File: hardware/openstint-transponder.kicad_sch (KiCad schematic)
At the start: 33 parts, among them J1 V+, J2 V-, Q1 AO3401A, U1 STM32C011F4Ux, U3 UCC27517DBV, U4 TLV760xx, Y1 20 MHz

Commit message: readme update
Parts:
- R3: LCSC (none) -> C17168
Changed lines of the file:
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@@
+			)
+		)
+		(property "LCSC" "C17168"
+			(at 180.34 140.97 90)
+			(effects
+				(font
+					(size 1.27 1.27)
+				)
+				(hide yes)
 			)
 		)

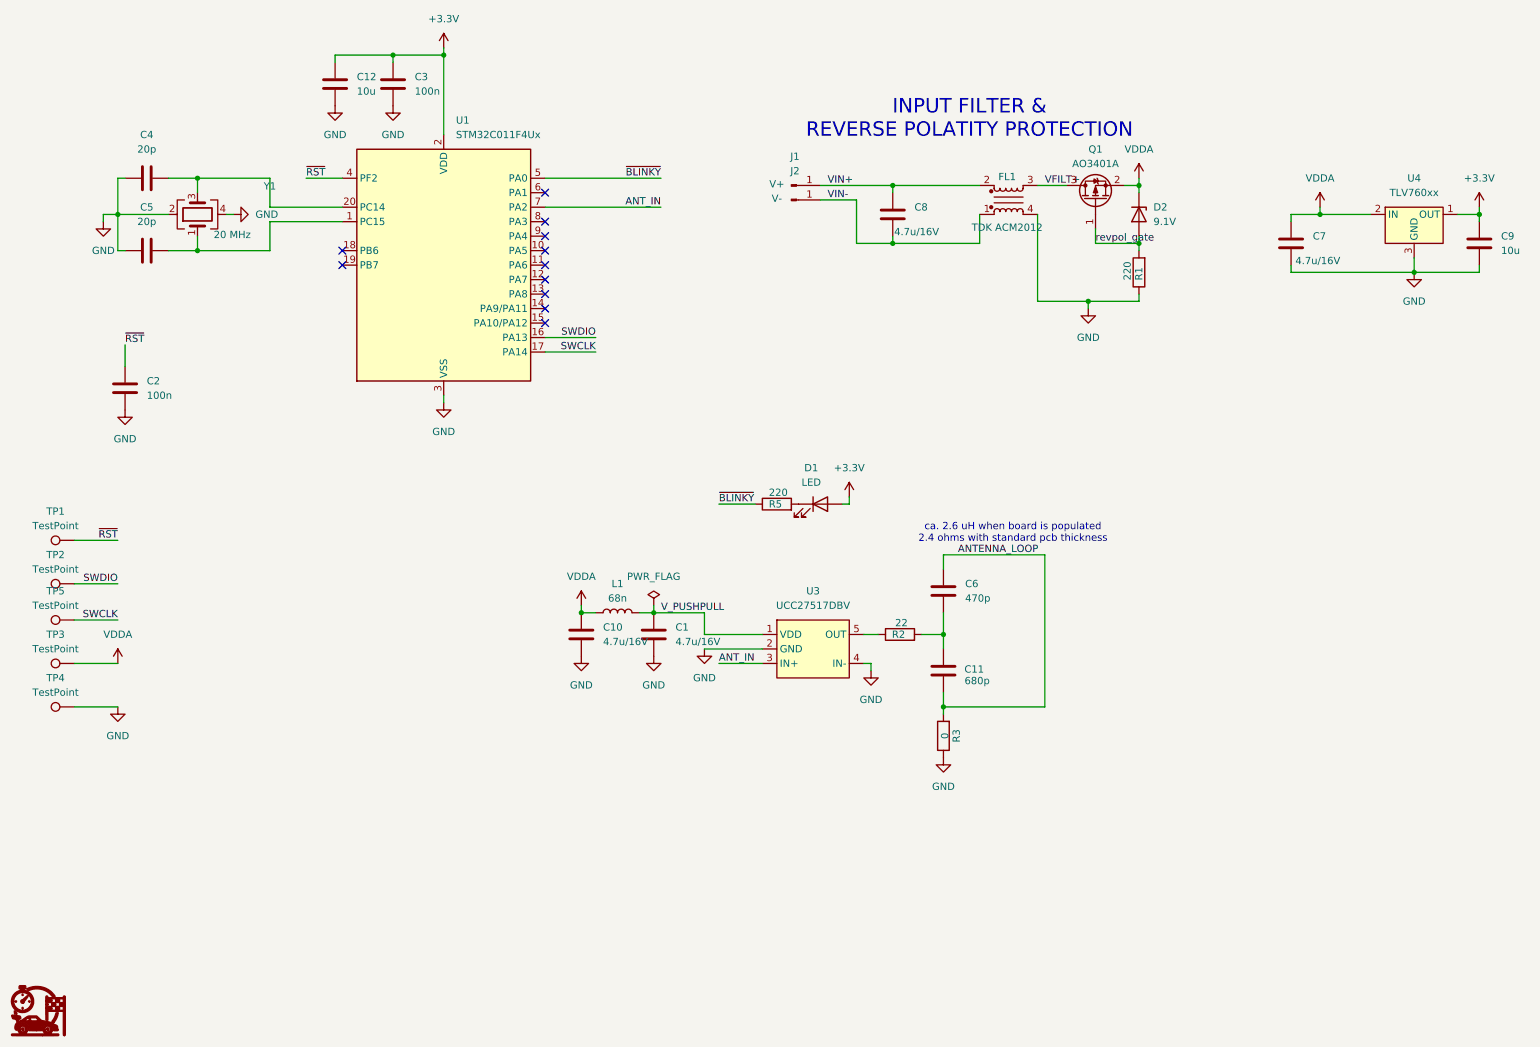
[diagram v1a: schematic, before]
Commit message: v2 transponder
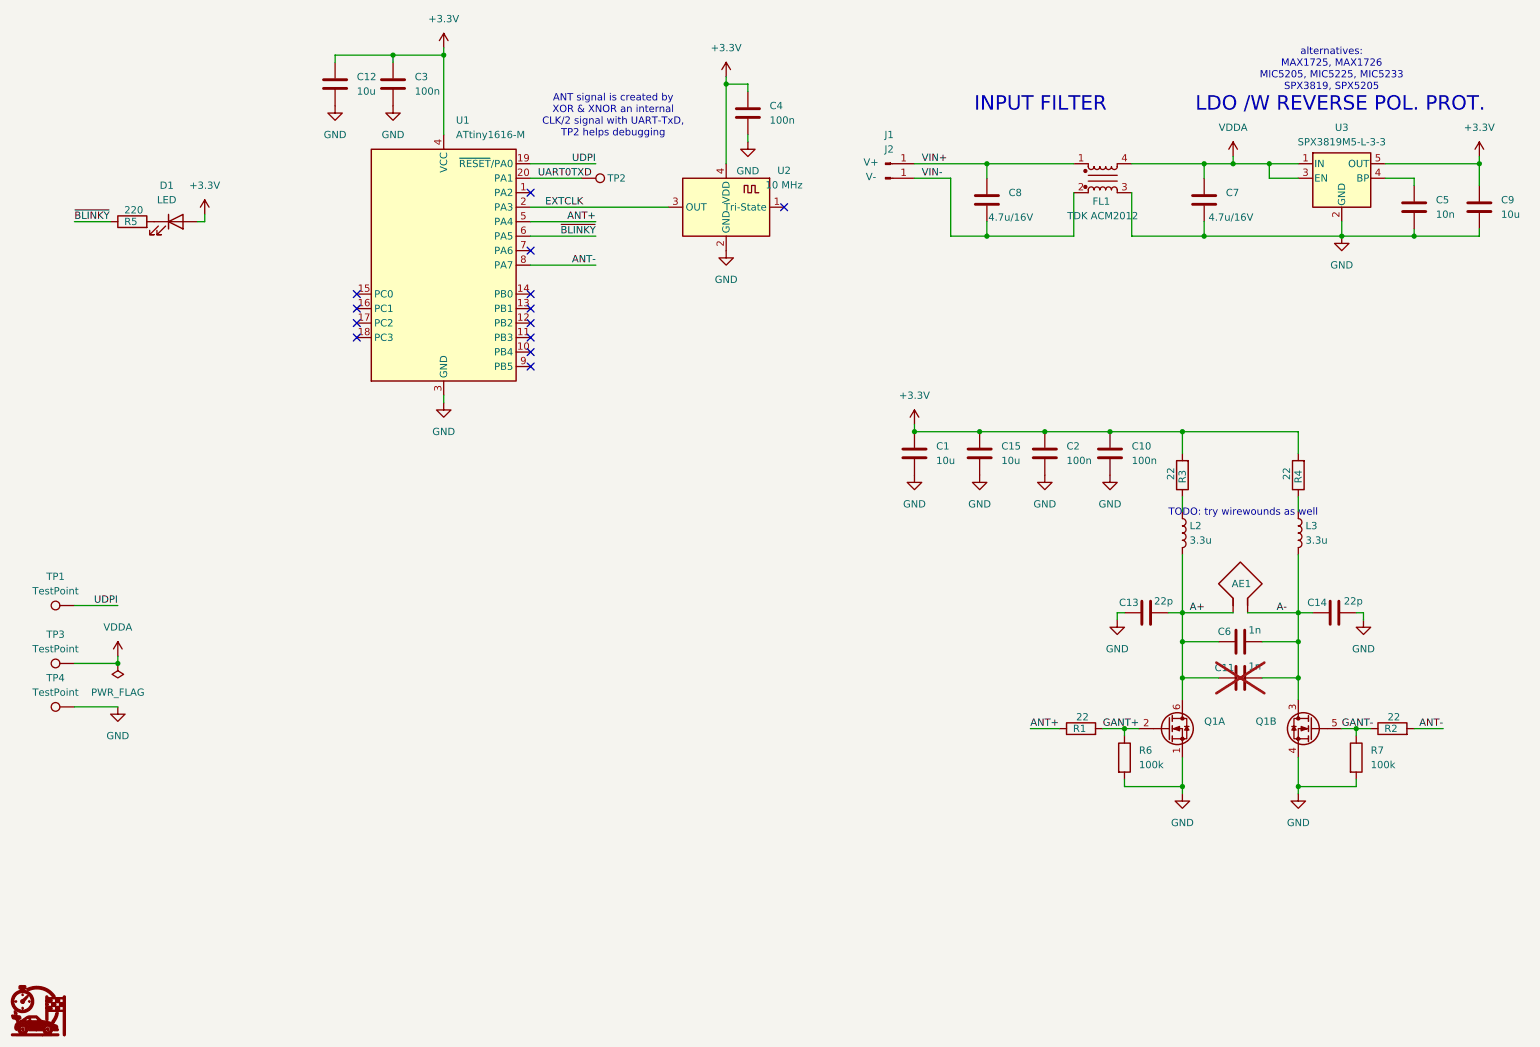
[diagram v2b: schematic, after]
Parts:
- removed D2: 9.1V, Diode_SMD:D_SOD-323, symbol Device:D_Zener
- removed L1: 68n, Inductor_SMD:L_0603_1608Metric, symbol Device:L
- removed Q1: AO3401A, Package_TO_SOT_SMD:SOT-23, symbol Transistor_FET:AO3401A
- removed TP5: TestPoint, TestPoint:TestPoint_Pad_D1.0mm, symbol Connector:TestPoint
- removed U1: STM32C011F4Ux, Package_DFN_QFN:ST_UFQFPN-20_3x3mm_P0.5mm, symbol MCU_ST_STM32C0:STM32C011F4Ux
- removed U3: UCC27517DBV, Package_TO_SOT_SMD:SOT-23-5, symbol Driver_FET:UCC27517DBV
- removed U4: TLV760xx, Package_TO_SOT_SMD:SOT-23, symbol Regulator_Linear:TLV760xx
- removed Y1: 20 MHz, Crystal:Crystal_SMD_3225-4Pin_3.2x2.5mm, symbol Device:Crystal_GND24
- added AE1: Antenna_Loop, symbol Device:Antenna_Loop
- added C13, C14: 22p, Capacitor_SMD:C_0402_1005Metric, symbol Device:C
- added C15: 10u, Capacitor_SMD:C_0402_1005Metric, symbol Device:C
- added L2, L3: 3.3u, Inductor_SMD:L_0603_1608Metric, symbol Device:L
- added Q1: PMGD280UN, Package_TO_SOT_SMD:SOT-363_SC-70-6, symbol Transistor_FET:Q_Dual_NMOS_S1G1D2S2G2D1
- added R4: 22, Resistor_SMD:R_0402_1005Metric, symbol Device:R
- added R6, R7: 100k, Resistor_SMD:R_0402_1005Metric, symbol Device:R
- added U1: ATtiny1616-M, Package_DFN_QFN:VQFN-20-1EP_3x3mm_P0.4mm_EP1.7x1.7mm, symbol MCU_Microchip_ATtiny:ATtiny1616-M
- added U2: 10 MHz, Crystal:Crystal_SMD_3225-4Pin_3.2x2.5mm, symbol symbols:Oscillator
- added U3: SPX3819M5-L-3-3, Package_TO_SOT_SMD:SOT-23-5, symbol Regulator_Linear:SPX3819M5-L-3-3
- C1: value 4.7u/16V -> 10u; footprint Capacitor_SMD:C_0603_1608Metric -> Capacitor_SMD:C_0402_1005Metric; LCSC C19666 -> C15525
- C10: value 4.7u/16V -> 100n; footprint Capacitor_SMD:C_0603_1608Metric -> Capacitor_SMD:C_0402_1005Metric; LCSC C19666 -> C1525
- C11: value 680p -> 1n; footprint Capacitor_SMD:C_0603_1608Metric -> Capacitor_SMD:C_0402_1005Metric; LCSC C30816 -> C1523; now not fitted
- C4: value 20p -> 100n; LCSC C1554 -> C1525
- C5: value 20p -> 10n; LCSC C1554 -> C15195
- C6: value 470p -> 1n; footprint Capacitor_SMD:C_0603_1608Metric -> Capacitor_SMD:C_0402_1005Metric; LCSC C1620 -> C1523
- R1: value 220 -> 22; LCSC C25091 -> C25092
- R3: value 0 -> 22; LCSC C17168 -> C25092
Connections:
- net VFILT+ is gone; now on net GND: FL1.3
- net V_PUSHPULL is gone; now on net +3.3V: C1.1
- net +3.3V: now also C10.2, C2.2, C4.2, R3.2, C15.1, R4.2, U1.4 (VCC), U2.4 (VDD), U3.5 (OUT)
- net GND: now also C10.1, C2.1, C5.2, C13.1, C14.2, C15.2, Q1.1 (S), Q1.4 (S), R6.2, R7.2, U1.21 (GND), U1.3 (GND), U2.2 (GND), U3.2 (GND); no longer C10.2, C2.2, C5.1, FL1.4, R1.1, R3.1
- net VDDA: now also FL1.4, U3.1 (IN), U3.3 (EN); no longer C10.1
- net VIN+: now also FL1.1; no longer FL1.2
- net VIN-: now also FL1.2; no longer FL1.1
- net ~{BLINKY}: now also U1.6 (PA5)
- net GANT-: now reaches R2.1
- net GANT-: now also Q1.5 (G), R7.1
- removed net ANTENNA_LOOP: C11.2, C6.1, R3.2
- net SWDIO renamed UART0TXD
- net UART0TXD: now also U1.20 (PA1)
- net revpol_gate renamed GANT+
- net GANT+: now also Q1.2 (G), R6.1
- net ~{RST} renamed UDPI
- net UDPI: now also U1.19 (~{RESET}/PA0); no longer C2.1
- new net: C5.1, U3.4 (BP)
- new net: L2.1, R3.1
- new net: L3.1, R4.1
- new net A+: AE1.1, C11.1, C13.2, C6.1, L2.2, Q1.6 (D)
- new net A-: AE1.2, C11.2, C14.1, C6.2, L3.2, Q1.3 (D)
- new net ANT+: R1.1, U1.5 (PA4)
- new net ANT-: R2.2, U1.8 (PA7)
- new net EXTCLK: U1.2 (PA3), U2.3 (OUT)
- no-connect marks 11 -> 13
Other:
- note added: "ANT signal is created by XOR & XNOR an internal CLK/2 signal with UART-TxD, TP2 helps debugging"
- note added: "INPUT FILTER"
- note added: "LDO /W REVERSE POL. PROT."
- note added: "TODO: try wirewounds as well"
- note added: "alternatives: MAX1725, MAX1726 MIC5205, MIC5225, MIC5233 SPX3819, SPX5205"
- note removed: "INPUT FILTER & REVERSE POLATITY PROTECTION"
- note removed: "ca. 2.6 uH when board is populated 2.4 ohms with standard pcb thickness"
- moved on the sheet: C7, C8, C9, D1, FL1, J1, J2, R5, TP1
